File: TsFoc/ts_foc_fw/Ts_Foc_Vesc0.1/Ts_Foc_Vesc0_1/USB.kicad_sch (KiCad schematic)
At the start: 6 parts

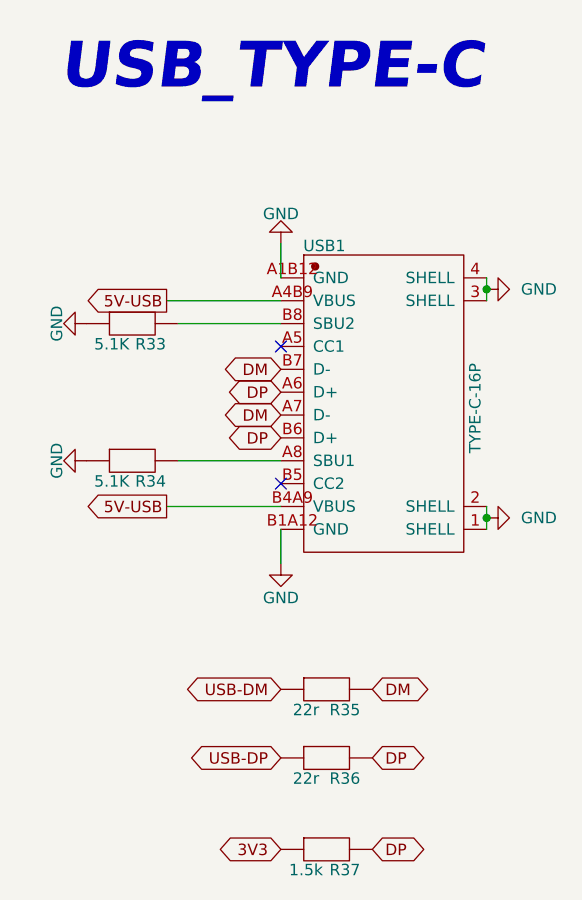
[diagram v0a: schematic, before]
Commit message: 电源走线完成
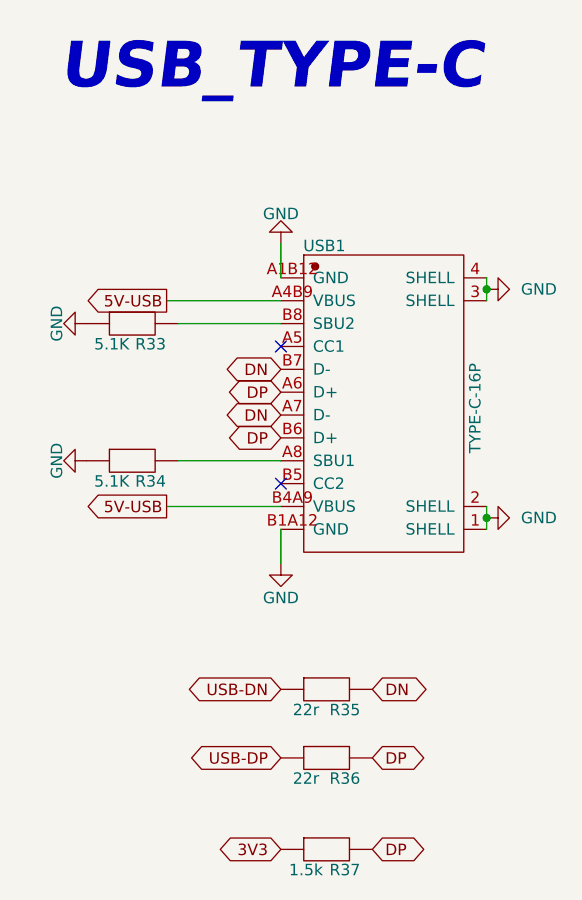
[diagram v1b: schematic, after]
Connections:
- net DM renamed DN
- net USB-DM renamed USB-DN
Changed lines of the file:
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@@
 		)
 	)
-	(global_label "DM"
+	(global_label "DN"
 		(shape bidirectional)
 		(at 148.59 95.25 180)
@@
 		)
 		(property "Intersheetrefs" "${INTERSHEET_REFS}"
-			(at 141.7721 95.25 0)
+			(at 141.893 95.25 0)
 			(effects
 				(font
@@
 		)
 	)
-	(global_label "USB-DM"
+	(global_label "USB-DN"
 		(shape bidirectional)
 		(at 148.59 130.81 180)
@@
 		)
 		(property "Intersheetrefs" "${INTERSHEET_REFS}"
-			(at 136.3897 130.81 0)
+			(at 136.5106 130.81 0)
 			(effects
 				(font
@@
 		)
 	)
-	(global_label "DM"
+	(global_label "DN"
 		(shape bidirectional)
 		(at 158.75 130.81 0)
@@
 		)
 		(property "Intersheetrefs" "${INTERSHEET_REFS}"
-			(at 165.5679 130.81 0)
+			(at 165.447 130.81 0)
 			(effects
 				(font
@@
 		)
 	)
-	(global_label "DM"
+	(global_label "DN"
 		(shape bidirectional)
 		(at 148.59 100.33 180)
@@
 		)
 		(property "Intersheetrefs" "${INTERSHEET_REFS}"
-			(at 141.7721 100.33 0)
-			(effects
-				(font
+			(at 141.893 100.33 0)
+			(effects
+				(font
